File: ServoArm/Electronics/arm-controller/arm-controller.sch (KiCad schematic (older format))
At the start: 1 part, among them U1 DRV11873

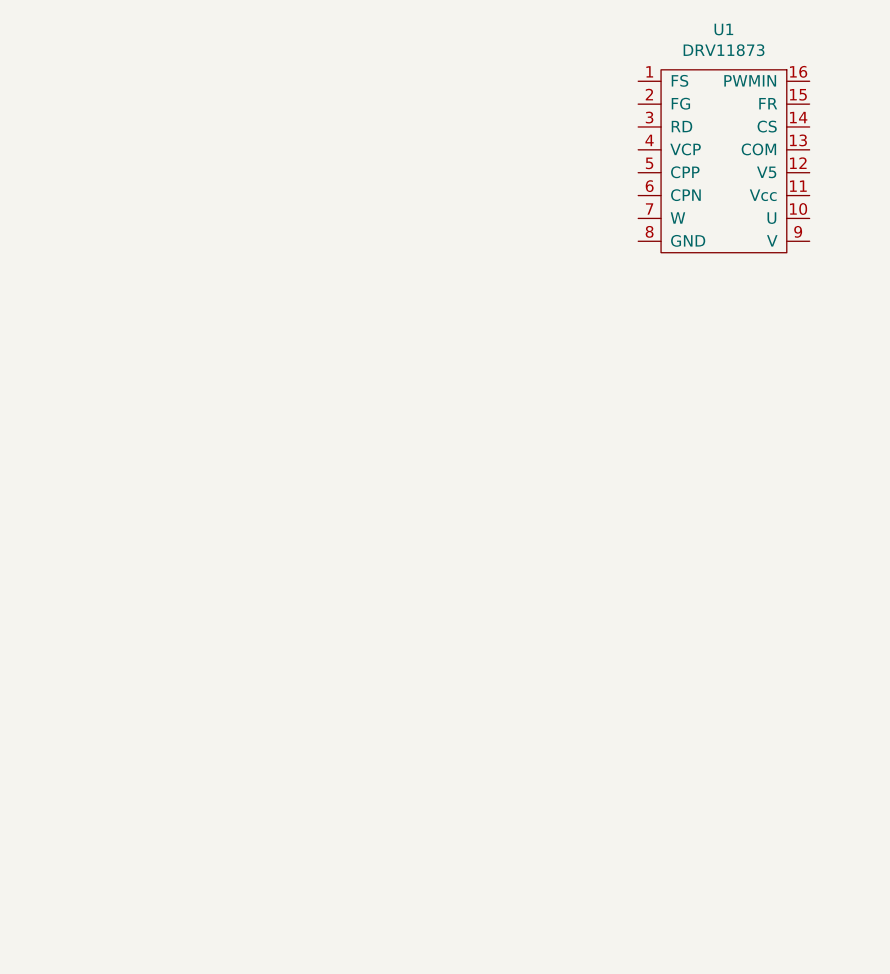
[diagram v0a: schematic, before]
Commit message: Arm WIP.
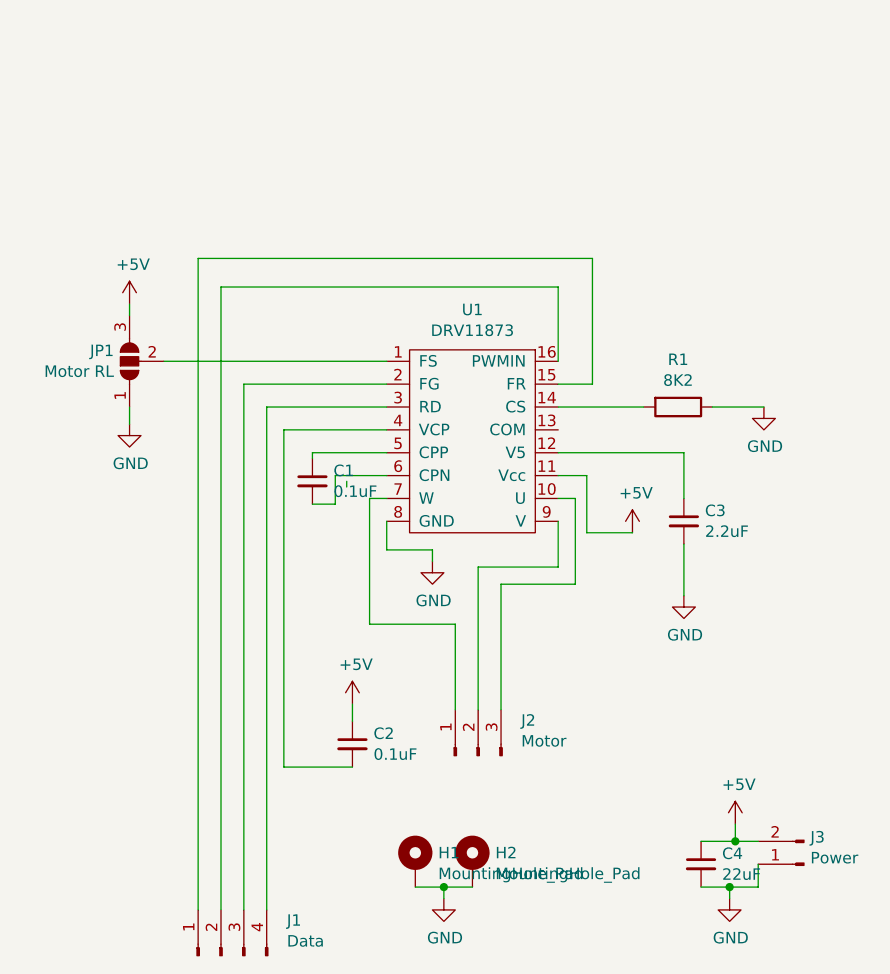
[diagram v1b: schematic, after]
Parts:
- added C1, C2: 0.1uF, Capacitor_SMD:C_0805_2012Metric, symbol Device:C_Small
- added C3: 2.2uF, Capacitor_SMD:C_0805_2012Metric, symbol Device:C_Small
- added C4: 22uF, Capacitor_SMD:C_0805_2012Metric, symbol Device:C_Small
- added H1, H2: MountingHole_Pad, MountingHole:MountingHole_2.7mm, symbol Mechanical:MountingHole_Pad
- added J1: Data, Connector_PinHeader_2.54mm:PinHeader_1x04_P2.54mm_Vertical, symbol Connector:Conn_01x04_Male
- added J2: Motor, Connector_PinHeader_2.54mm:PinHeader_1x03_P2.54mm_Vertical, symbol Connector:Conn_01x03_Male
- added J3: Power, Connector_PinHeader_2.54mm:PinHeader_1x02_P2.54mm_Vertical, symbol Connector:Conn_01x02_Male
- added JP1: Motor RL, Jumper:SolderJumper-3_P1.3mm_Open_Pad1.0x1.5mm, symbol Jumper:SolderJumper_3_Open
- added R1: 8K2, Resistor_SMD:R_0805_2012Metric, symbol Device:R
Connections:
- net labels added: +5V, GND
- wire segments 0 -> 56
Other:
- moved on the sheet: U1
